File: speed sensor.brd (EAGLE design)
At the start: 69.8 x 73.3 mm, 11 parts, among them IC1 LM358N

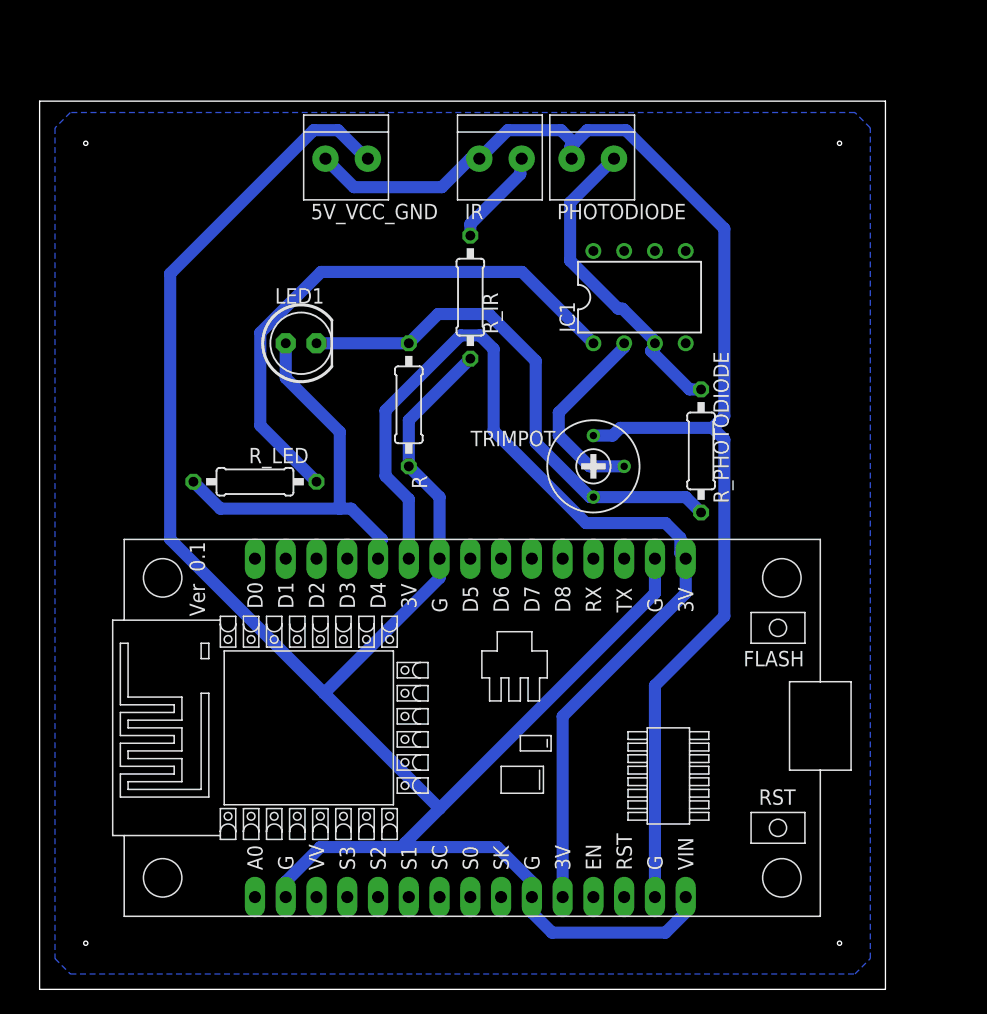
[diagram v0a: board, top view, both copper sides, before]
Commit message: board rev 5
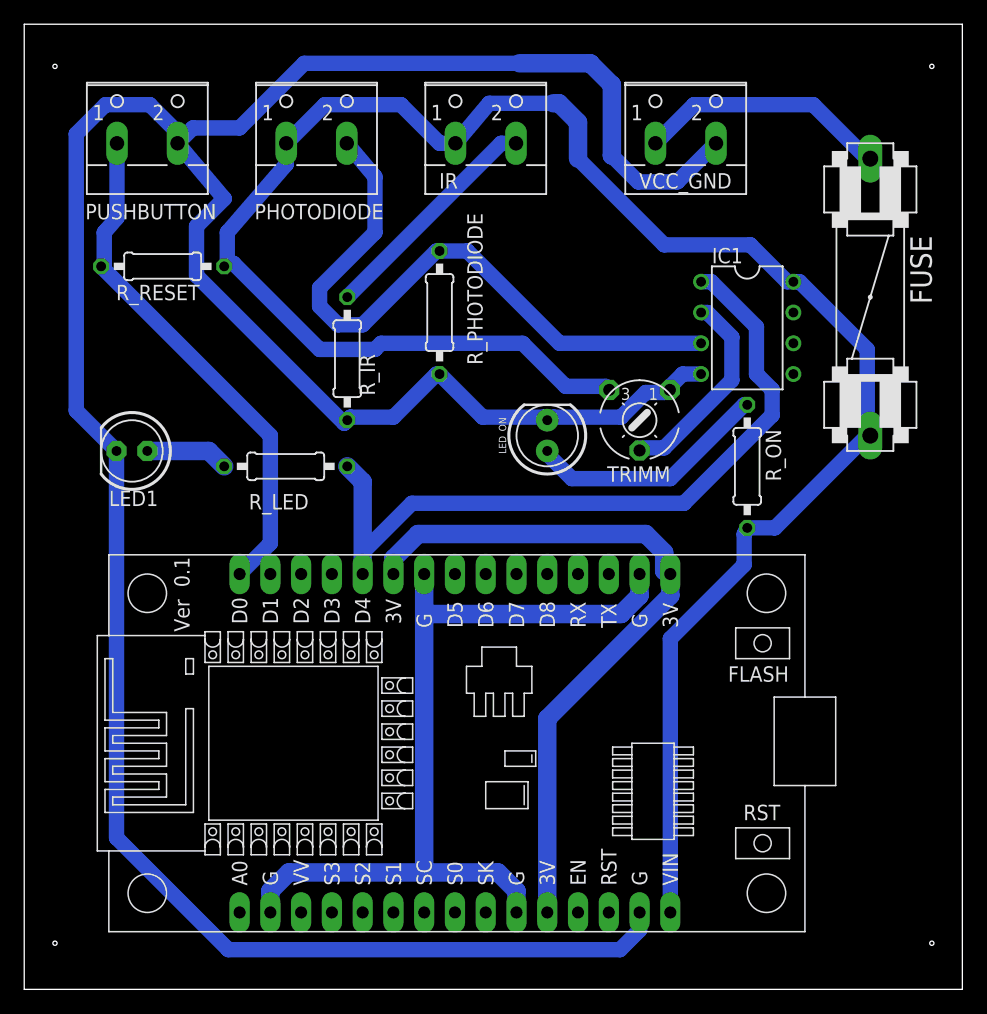
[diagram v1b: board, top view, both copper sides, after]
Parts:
- removed 5V_VCC_GND: 1X2-3.5MM, adafruit:1X2-3.5MM
- removed R: 68K, rcl:0207/10
- removed TRIMPOT: 10k, rcl:RTRIM3339P
- added FUSE: 1 amp, special:FUSE
- added LED_ON: (no value), SparkFun-LED:LED_5MM
- added PUSHBUTTON, VCC_GND: (no value), con-wago-500:W237-102
- added R_ON: 330, rcl:0207/10
- added R_RESET: 10k, rcl:0207/10
- added TRIMM: 10k, adafruit:6MM
- IR, PHOTODIODE: value 1X2-3.5MM -> (none); device adafruit:1X2-3.5MM -> con-wago-500:W237-102
- moved R_PHOTODIODE 24.4 mm to (26.7, 86.4)
- moved PHOTODIODE 23.0 mm to (16.5, 101.6), turned to 0 degrees
- moved LED1 16.6 mm to (1.27, 74.9), turned to 180 degrees
- moved R_IR 11.4 mm to (19.1, 82.5)
- moved IC1 9.25 mm to (52.1, 85.1), turned to 270 degrees
- moved R_LED 2.84 mm to (14.0, 73.7)
- moved IR 2.84 mm to (30.5, 101.6), turned to 0 degrees
- moved U$1 1.80 mm to (27.9, 50.8)
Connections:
- removed net N$5: LED1.K, R.1, R_PHOTODIODE.1, TRIMPOT.1
- removed net N$7: IC1.1, R_LED.2
- removed net V+: IC1.8
- removed net V-: IC1.4
- new net GND: IC1.4, LED1.K, LED_ON.K, PUSHBUTTON.2, R_IR.1, R_PHOTODIODE.1, TRIMM.A, U$1.14, VCC_GND.2
- new net N$10: LED_ON.A, R_ON.1
- new net N$13: FUSE.2, IC1.8, IR.1, PHOTODIODE.1, R_ON.2, R_RESET.1, TRIMM.E, U$1.15
- new net N$9: PUSHBUTTON.1, R_RESET.2, U$1.30
- new net VCC: FUSE.1, VCC_GND.1
- net N$1: now also LED1.A, R_LED.1; no longer 5V_VCC_GND.1, IR.1, PHOTODIODE.1, TRIMPOT.3, U$1.14
- net N$3: no longer 5V_VCC_GND.2, R.2, R_IR.1, U$1.15
- net N$6: now also TRIMM.S; no longer TRIMPOT.2
- net N$8: now also IC1.1, R_LED.2; no longer LED1.A, R_LED.1
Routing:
- net GND: track 0.00 -> 240.7 mm
- net N$13: track 0.00 -> 165.5 mm
- net N$3: track 184.5 -> 70.0 mm
- net N$1: track 110.1 -> 6.88 mm
- net N$7: track 46.2 -> 0.00 mm
- net N$5: track 43.5 -> 0.00 mm
- net N$9: track 0.00 -> 42.9 mm
- net N$8: track 34.8 -> 63.6 mm
- net N$4: track 26.1 -> 54.0 mm
- net 3V: track 84.9 -> 59.3 mm
- net VCC: track 0.00 -> 20.9 mm
- net N$10: track 0.00 -> 20.1 mm
- net N$2: track 8.17 -> 19.2 mm
- net N$6: track 16.3 -> 17.1 mm
- removed copper zone on layer 16, net BOTOM
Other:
- board size 69.8 x 73.3 mm -> 77.5 x 79.7 mm
